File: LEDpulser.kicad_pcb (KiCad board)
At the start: 2 copper layers, 38.2 x 98.2 mm, 63 parts, among them J1 RJHSE5380, J2 EPS.00.250.NTN, J3 EPS.00.250.NTN, J4 Conn_01x04_Female, J5 LED, Q1 AO3401A, Q2 AO3400A, Q3 AO3400A, SW1 BST11T2AVR, U1 74HC123, U10 LT3082, U2 74HC123, U3 74HC123, U4 74HC10, U5 LT1121-5, U6 PM8834, U7 NE555, U8 PM8834, U9 PM8834

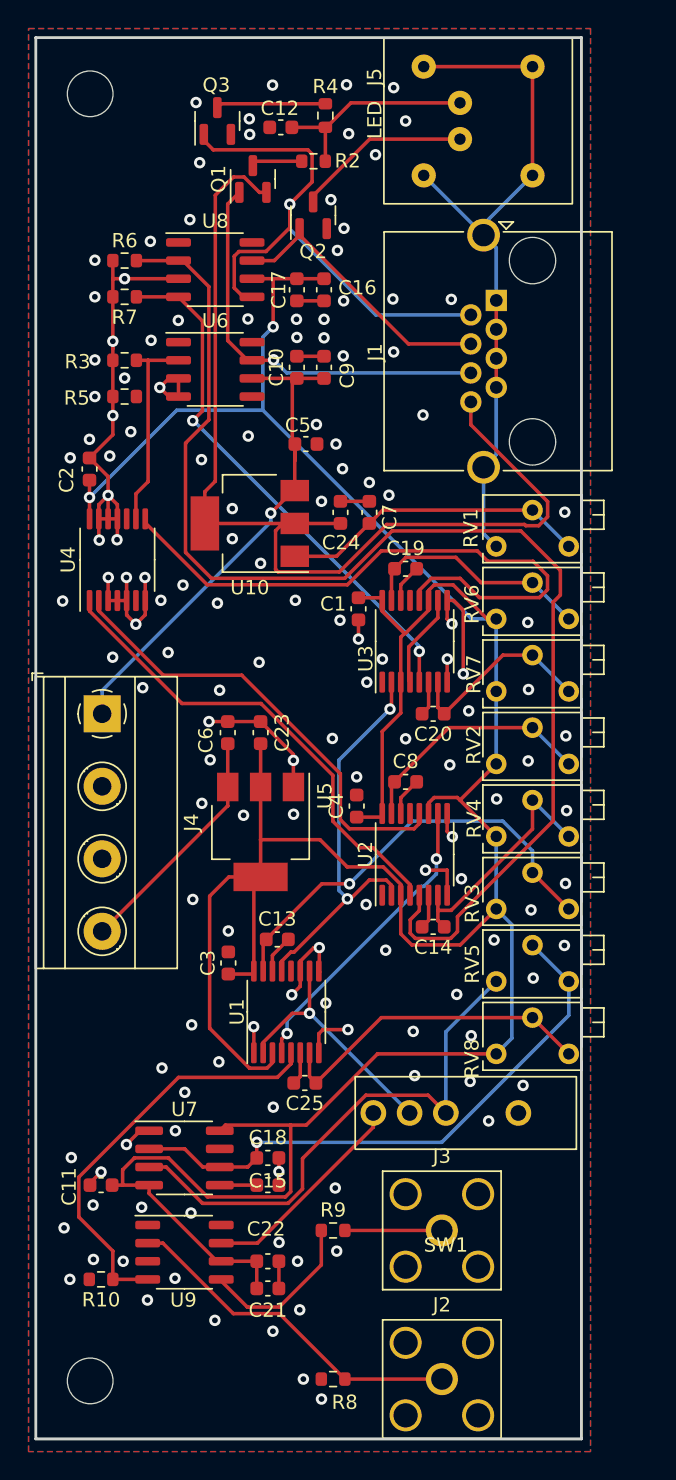
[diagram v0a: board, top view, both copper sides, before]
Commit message: reverted to previous commit
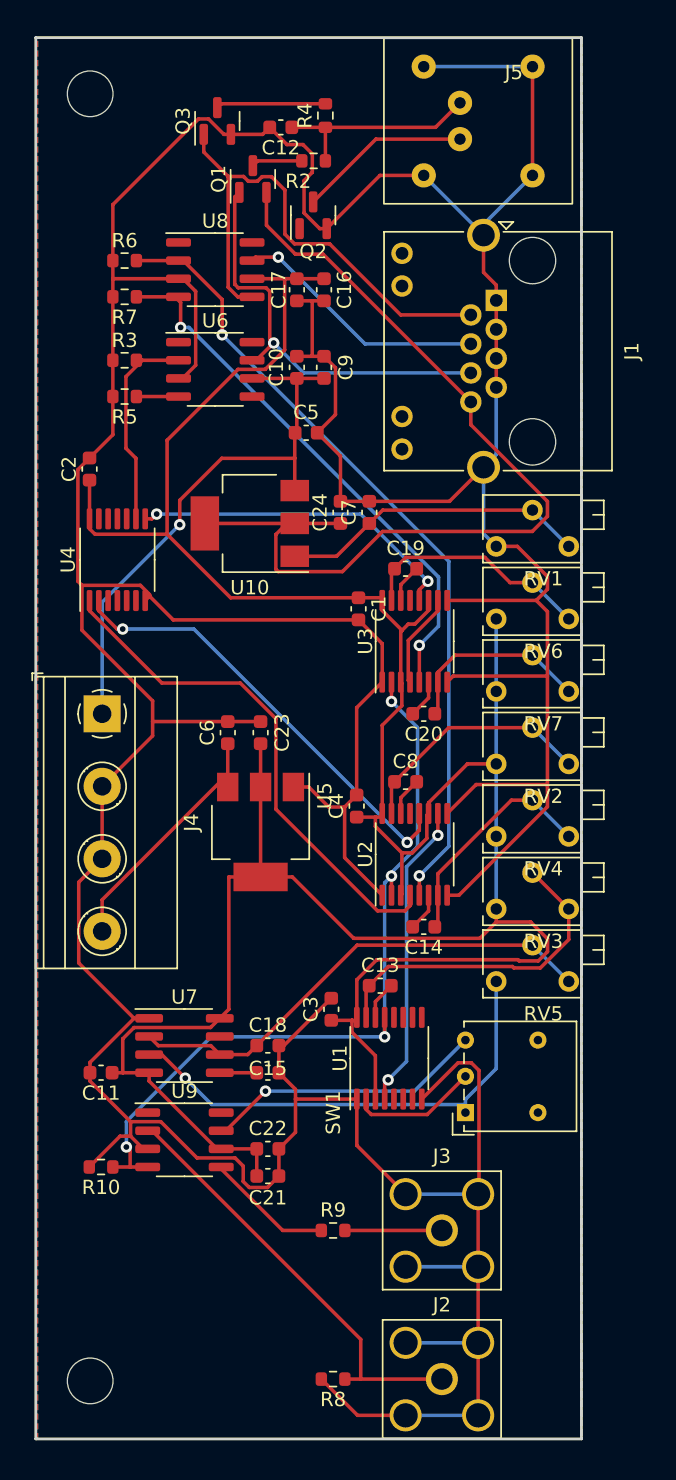
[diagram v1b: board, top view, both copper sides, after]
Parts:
- removed C25: C, Capacitor_SMD:C_0603_1608Metric
- removed RV8: 2k, Potentiometer_THT:Potentiometer_Bourns_3266X_Horizontal
- J1: value RJHSE5380 -> RJ45_Shielded; footprint Connector_RJ:RJ45_Amphenol_RJHSE5380 -> Connector_RJ:RJ45_Amphenol_RJHSE538X
- R8: value 100k -> 50
- SW1: value BST11T2AVR -> ATE1D-5M3-10-Z
- moved C3 7.91 mm to (122.2, 93.5)
- moved C13 7.91 mm to (125.6, 91.8)
- moved U1 7.91 mm to (126.2, 96.9)
- moved C11 7.87 mm to (106.0, 97.9)
- moved C15 7.87 mm to (117.7, 97.9)
- moved C18 7.87 mm to (117.7, 96.0)
- moved C21 7.87 mm to (117.7, 105.2)
- moved C22 7.87 mm to (117.7, 103.3)
- moved R10 7.87 mm to (106.0, 104.5)
- moved U7 7.87 mm to (111.9, 96.0)
- moved U9 7.87 mm to (111.9, 102.6)
- moved SW1 1.37 mm to (131.6, 100.7), turned to 90 degrees
- moved C5 0.79 mm to (120.4, 53.1)
- moved C14 0.66 mm to (128.7, 87.7)
- moved C20 0.66 mm to (128.7, 72.8)
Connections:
- Q2 pad 1: /LED_ON -> unconnected-(Q2-Pad1)
- U1 pad 10: Net-(SW1-Pad2) -> (no net)
- U1 pad 11: GND -> (no net)
- U1 pad 12: unconnected-(U1-Pad12) -> (no net)
- U1 pad 13: Net-(U1-Pad13) -> Net-(R10-Pad1)
- U1 pad 5: Net-(R10-Pad1) -> (no net)
- U1 pad 6: Net-(C25-Pad2) -> (no net)
- U1 pad 7: Net-(C25-Pad1) -> (no net)
- U1 pad 9: GND -> (no net)
- U2 pad 2: Net-(U1-Pad13) -> Net-(R10-Pad1)
- U3 pad 2: Net-(U1-Pad13) -> Net-(R10-Pad1)
- U4 pad 10: unconnected-(U4-Pad10) -> (no net)
- U4 pad 11: GND -> (no net)
- U4 pad 12: GND -> (no net)
- U4 pad 13: GND -> (no net)
- U4 pad 3: GND -> (no net)
- U4 pad 4: GND -> (no net)
- U4 pad 5: GND -> (no net)
- U4 pad 6: unconnected-(U4-Pad6) -> (no net)
- U6 pad 4: GND -> Net-(R5-Pad1)
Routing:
- net GND: track 145.5 -> 410.9 mm, vias 146 -> 0
- net Net-(R6-Pad1): track 89.5 -> 56.3 mm, vias 0 -> 2
- net +5V: track 236.6 -> 207.9 mm, vias 2 -> 0
- net Net-(U1-Pad13): track 28.5 -> 0.00 mm, vias 2 -> 0
- net Net-(R10-Pad1): track 29.5 -> 55.6 mm, vias 0 -> 4
- net Net-(C25-Pad1): track 23.4 -> 0.00 mm
- net Net-(U3-Pad12): track 43.8 -> 23.5 mm, vias 0 -> 2
- net Net-(SW1-Pad2): track 17.7 -> 8.94 mm, vias 1 -> 0
- net Net-(C13-Pad1): track 30.4 -> 23.4 mm, vias 1 -> 0
- net Net-(C18-Pad1): track 40.9 -> 34.2 mm, vias 1 -> 0
- net /CAP_VOLTAGE: track 71.9 -> 65.7 mm
- net /EXT: track 24.6 -> 30.6 mm
- net Net-(SW1-Pad3): track 15.0 -> 19.7 mm, vias 0 -> 1
- net +12V: track 35.4 -> 39.5 mm
- net /INT: track 37.4 -> 33.7 mm, vias 0 -> 1
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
